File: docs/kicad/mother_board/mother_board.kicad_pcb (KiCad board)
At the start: 2 copper layers, 18 parts, among them J1 EXPR, J2 TFT_CONTROL, J3 TFT_DATA, J4 SERIAL, J5 LEDS, J6 ROTARY12, J7 ROTARY34, J8 SW_OUT, J9 SW_IN, U1 myTeensy3.6

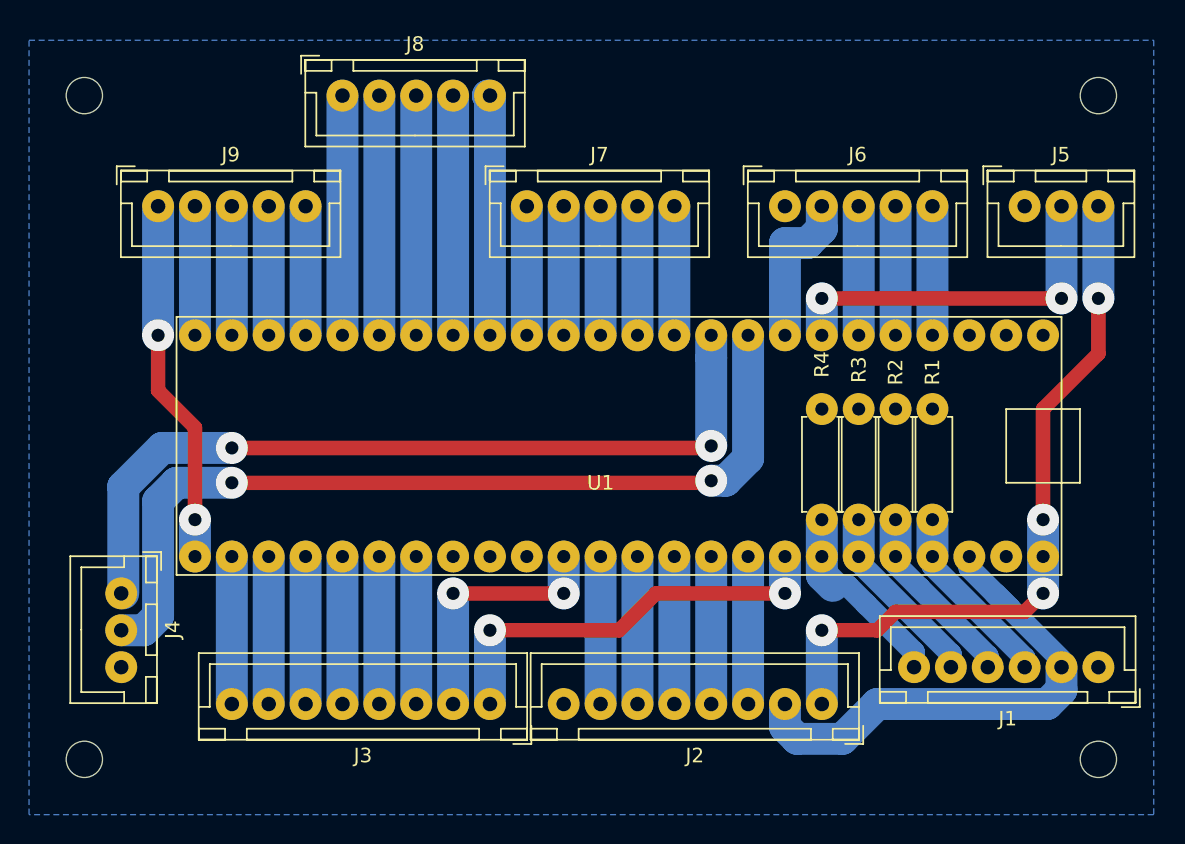
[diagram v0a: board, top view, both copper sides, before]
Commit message: start MAKE NEW motherboard and display_connector FOR olds TeensyExprssion box with TE2 code
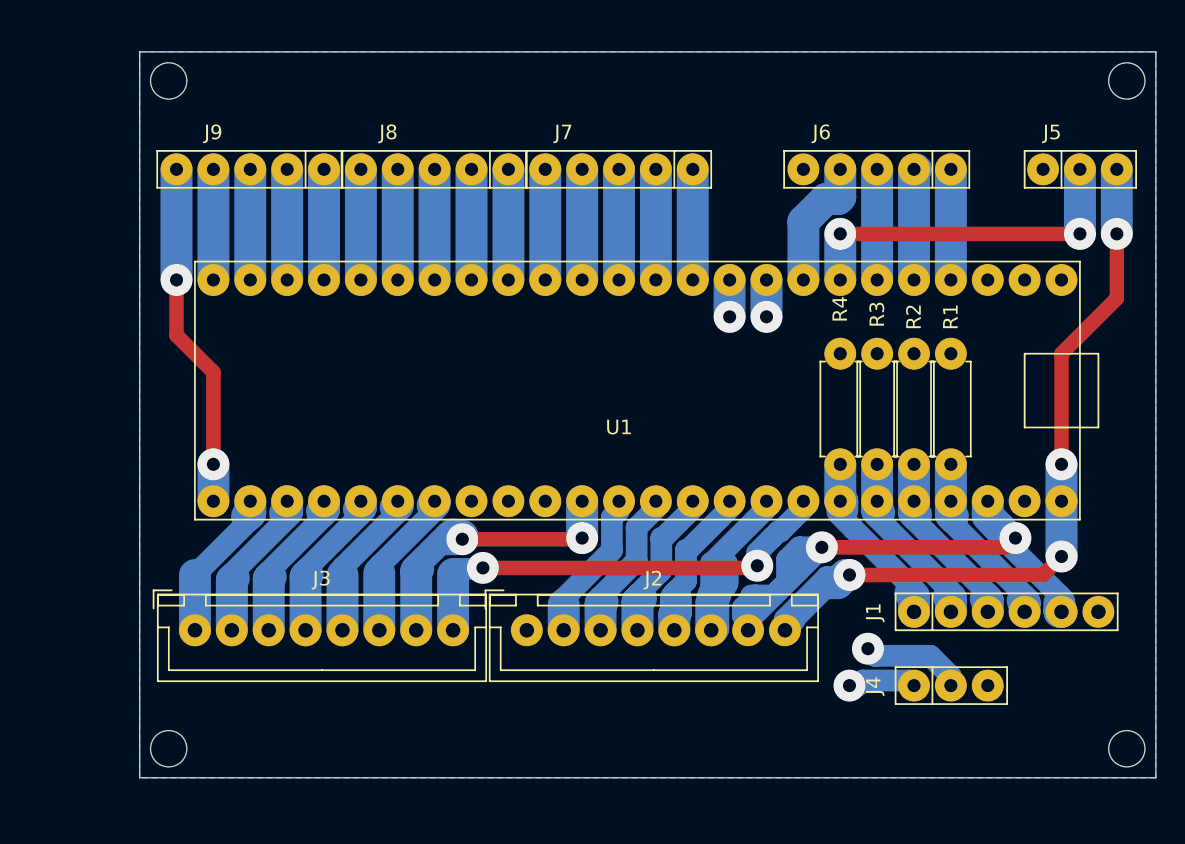
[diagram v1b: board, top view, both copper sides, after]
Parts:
- removed the REF** at (-3.81, -47.0)
- removed the REF** at (66.0, -1.27)
- removed the REF** at (66.0, -47.0)
- added REF**: myMountingHole_2.5mm, 0_my_footprints:myMountingHole_2.5mm, F.Cu at (2.00, -48.0)
- added REF**: myMountingHole_2.5mm, 0_my_footprints:myMountingHole_2.5mm, F.Cu at (68.0, -2.00)
- added REF**: myMountingHole_2.5mm, 0_my_footprints:myMountingHole_2.5mm, F.Cu at (68.0, -48.0)
- J1: footprint 0_my_footprints:myJSTx06 -> 0_my_footprints:myPinSocket_1x06
- J4, J5: footprint 0_my_footprints:myJSTx03 -> 0_my_footprints:myPinSocket_1x03
- J6, J7, J8, J9: footprint 0_my_footprints:myJSTx05 -> 0_my_footprints:myPinSocket_1x05
- moved J4 55.0 mm to (53.3, -6.35), turned to 90 degrees
- moved J2 20.9 mm to (26.7, -10.2), turned to 0 degrees
- moved J3 20.9 mm to (3.81, -10.2), turned to 0 degrees
- moved J1 13.3 mm to (53.3, -11.4), turned to 90 degrees
- moved J8 12.5 mm to (25.4, -41.9), turned to 270 degrees
- moved J6 11.7 mm to (55.9, -41.9), turned to 270 degrees
- moved J7 11.7 mm to (38.1, -41.9), turned to 270 degrees
- moved J9 11.7 mm to (12.7, -41.9), turned to 270 degrees
- moved REF** 5.86 mm to (2.00, -2.00)
- moved U1 4.02 mm to (34.3, -26.7)
- moved R1 4.02 mm to (55.9, -21.6)
- moved R2 4.02 mm to (53.3, -21.6)
- moved R3 4.02 mm to (50.8, -21.6)
- moved R4 4.02 mm to (48.3, -21.6)
- moved J5 2.84 mm to (62.2, -41.9), turned to 90 degrees
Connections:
- J1 pad 1: GND -> EXPR4
- J1 pad 2: +3V3 -> EXPR3
- J1 pad 3: EXPR1 -> EXPR2
- J1 pad 4: EXPR2 -> EXPR1
- J1 pad 5: EXPR3 -> +3V3
- J1 pad 6: EXPR4 -> GND
- J2 pad 1: +5V -> GND
- J2 pad 2: +3V3 -> TFT_RD
- J2 pad 3: TFT_RES -> TFT_WR
- J2 pad 4: TFT_CS -> TFT_CD_RS
- J2 pad 5: TFT_CD_RS -> TFT_CS
- J2 pad 6: TFT_WR -> TFT_RES
- J2 pad 7: TFT_RD -> +3V3
- J2 pad 8: GND -> +5V
- J3 pad 1: TFT_DAT1 -> TFT_DAT2
- J3 pad 2: TFT_DAT0 -> TFT_DAT3
- J3 pad 3: TFT_DAT7 -> TFT_DAT4
- J3 pad 4: TFT_DAT6 -> TFT_DAT5
- J3 pad 5: TFT_DAT5 -> TFT_DAT6
- J3 pad 6: TFT_DAT4 -> TFT_DAT7
- J3 pad 7: TFT_DAT3 -> TFT_DAT0
- J3 pad 8: TFT_DAT2 -> TFT_DAT1
- J6 pad 1: GND -> ROT1A
- J6 pad 2: ROT2A -> ROT1B
- J6 pad 3: ROT2B -> ROT2A
- J6 pad 4: ROT1B -> ROT2B
- J6 pad 5: ROT1A -> GND
- J7 pad 1: +3V3 -> ROT3A
- J7 pad 2: ROT4A -> ROT3B
- J7 pad 3: ROT4B -> ROT4A
- J7 pad 4: ROT3B -> ROT4B
- J7 pad 5: ROT3A -> +3V3
- J8 pad 1: SW_OUT5 -> SW_OUT0
- J8 pad 2: SW_OUT4 -> SW_OUT1
- J8 pad 3: SW_OUT3 -> SW_OUT2
- J8 pad 4: SW_OUT2 -> SW_OUT3
- J8 pad 5: SW_OUT1 -> SW_OUT4
- J9 pad 1: SW_IN5 -> SW_IN0
- J9 pad 2: SW_IN4 -> SW_IN1
- J9 pad 3: SW_IN3 -> SW_IN2
- J9 pad 4: SW_IN2 -> SW_IN3
- J9 pad 5: SW_IN1 -> SW_IN4
- U1 pad 13: ROT4B -> ROT4A
- U1 pad 14: ROT4A -> ROT4B
- U1 pad 16: SW_OUT1 -> SW_OUT0
- U1 pad 17: SW_OUT2 -> SW_OUT1
- U1 pad 18: SW_OUT3 -> SW_OUT2
- U1 pad 19: SW_OUT4 -> SW_OUT3
- U1 pad 20: SW_OUT5 -> SW_OUT4
- U1 pad 21: SW_IN1 -> SW_IN0
- U1 pad 22: SW_IN2 -> SW_IN1
- U1 pad 23: SW_IN3 -> SW_IN2
- U1 pad 24: SW_IN4 -> SW_IN3
- U1 pad 25: SW_IN5 -> SW_IN4
- U1 pad 6: ROT2B -> ROT2A
- U1 pad 8: ROT2A -> ROT2B
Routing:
- net RX3: track 61.2 -> 9.68 mm
- net TX3: track 56.6 -> 7.27 mm
- net SW_IN5: track 25.2 -> 0.00 mm, vias 2 -> 0
- net SW_OUT5: track 16.5 -> 0.00 mm
- net SW_IN4: track 8.89 -> 23.9 mm, vias 0 -> 2
- net SW_OUT1: track 16.7 -> 7.62 mm
- net SW_OUT4: track 16.5 -> 7.62 mm
- net SW_OUT3: track 16.5 -> 7.62 mm
- net SW_OUT2: track 16.5 -> 7.62 mm
- net SW_OUT0: track 0.00 -> 7.62 mm
- net SW_IN0: track 0.00 -> 7.62 mm
- net +3V3: track 44.0 -> 51.6 mm, vias 0 -> 2
- net +5V: track 49.6 -> 55.8 mm
- net TFT_RES: track 10.2 -> 15.3 mm
- net TFT_DAT3: track 10.2 -> 15.0 mm
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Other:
- board outline added: 70 x 50 mm
